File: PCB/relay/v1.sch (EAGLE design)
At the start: 7 parts, among them T1 BC817, U1 SFH615A-07, U2 ALQ105

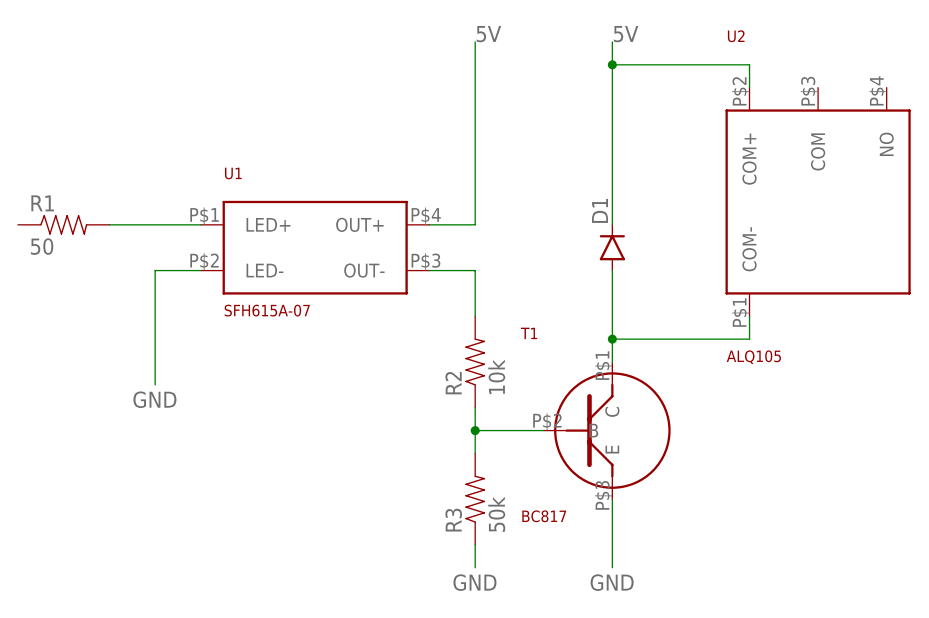
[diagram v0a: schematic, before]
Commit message: Adding files for v0.2
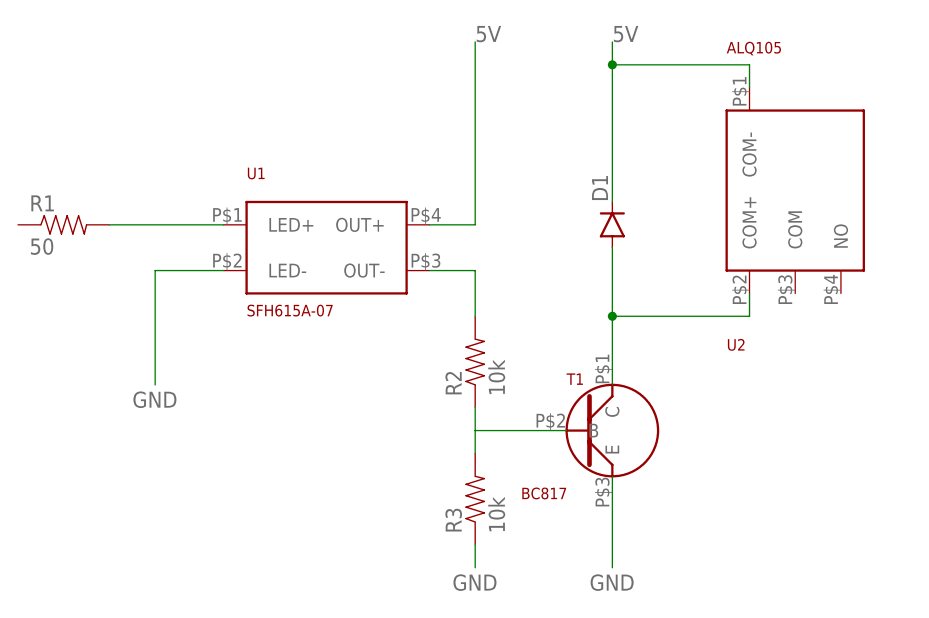
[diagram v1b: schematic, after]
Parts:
- R3: value 50k -> 10k
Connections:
- net 5V: now also U2.COM-; no longer U2.COM+
- net N$4: now also U2.COM+; no longer U2.COM-
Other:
- moved on the sheet: D1, U1, U2
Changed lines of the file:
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@@
 </classes>
 <parts>
-<part name="U1" library="lib" deviceset="SFH615A-07" device=""/>
+<part name="U1" library="lib" library_urn="urn:adsk.eagle:library:473707" deviceset="SFH615A-07" device="" package3d_urn="urn:adsk.eagle:package:473718/1"/>
 <part name="R1" library="SparkFun-Passives" deviceset="RESISTOR" device="0603-RES" value="50"/>
-<part name="T1" library="lib" deviceset="BC817" device=""/>
+<part name="T1" library="lib" library_urn="urn:adsk.eagle:library:473707" deviceset="BC817" device="" package3d_urn="urn:adsk.eagle:package:473719/1"/>
 <part name="R2" library="SparkFun-Passives" deviceset="RESISTOR" device="0603-RES" value="10k"/>
-<part name="R3" library="SparkFun-Passives" deviceset="RESISTOR" device="0603-RES" value="50k"/>
 <part name="D1" library="SparkFun-DiscreteSemi" deviceset="DIODE" device="SMA"/>
-<part name="U2" library="lib" deviceset="ALQ105" device=""/>
+<part name="U2" library="lib" library_urn="urn:adsk.eagle:library:473707" deviceset="ALQ105" device="" package3d_urn="urn:adsk.eagle:package:473720/1"/>
+<part name="R3" library="SparkFun-Passives" deviceset="RESISTOR" device="0603-RES" value="10k"/>
 </parts>
 <sheets>
@@
 <instance part="U1" gate="G$1" x="40.64" y="48.26"/>
 <instance part="R1" gate="G$1" x="12.7" y="50.8"/>
-<instance part="T1" gate="G$1" x="73.66" y="27.94"/>
+<instance part="T1" gate="G$1" x="73.66" y="27.94" smashed="yes">
+<attribute name="NAME" x="68.58" y="33.02" size="1.27" layer="94"/>
+<attribute name="VALUE" x="63.5" y="20.32" size="1.27" layer="94"/>
+</instance>
 <instance part="R2" gate="G$1" x="58.42" y="35.56" rot="R90"/>
+<instance part="D1" gate="G$1" x="73.66" y="50.8" rot="R90"/>
+<instance part="U2" gate="G$1" x="93.98" y="53.34" rot="MR180"/>
 <instance part="R3" gate="G$1" x="58.42" y="20.32" rot="R90"/>
-<instance part="D1" gate="G$1" x="73.66" y="48.26" rot="R90"/>
-<instance part="U2" gate="G$1" x="106.68" y="48.26"/>
 </instances>
 <busses>
@@
 <pinref part="R1" gate="G$1" pin="2"/>
 <pinref part="U1" gate="G$1" pin="LED+"/>
-<wire x1="17.78" y1="50.8" x2="27.94" y2="50.8" width="0.1524" layer="91"/>
+<wire x1="17.78" y1="50.8" x2="30.48" y2="50.8" width="0.1524" layer="91"/>
 </segment>
 </net>
@@
 <segment>
 <pinref part="U1" gate="G$1" pin="LED-"/>
-<wire x1="27.94" y1="45.72" x2="22.86" y2="45.72" width="0.1524" layer="91"/>
+<wire x1="30.48" y1="45.72" x2="22.86" y2="45.72" width="0.1524" layer="91"/>
 <wire x1="22.86" y1="45.72" x2="22.86" y2="33.02" width="0.1524" layer="91"/>
 <label x="20.32" y="30.48" size="1.778" layer="95"/>
+</segment>
+<segment>
+<pinref part="T1" gate="G$1" pin="E"/>
+<wire x1="73.66" y1="22.86" x2="73.66" y2="12.7" width="0.1524" layer="91"/>
+<label x="71.12" y="10.16" size="1.778" layer="95"/>
 </segment>
 <segment>
@@
 <wire x1="58.42" y1="15.24" x2="58.42" y2="12.7" width="0.1524" layer="91"/>
 <label x="55.88" y="10.16" size="1.778" layer="95"/>
-</segment>
-<segment>
-<pinref part="T1" gate="G$1" pin="E"/>
-<wire x1="73.66" y1="20.32" x2="73.66" y2="12.7" width="0.1524" layer="91"/>
-<label x="71.12" y="10.16" size="1.778" layer="95"/>
 </segment>
 </net>
@@
 <segment>
 <pinref part="R2" gate="G$1" pin="1"/>
-<pinref part="R3" gate="G$1" pin="2"/>
 <wire x1="58.42" y1="30.48" x2="58.42" y2="27.94" width="0.1524" layer="91"/>
 <pinref part="T1" gate="G$1" pin="B"/>
+<wire x1="68.58" y1="27.94" x2="58.42" y2="27.94" width="0.1524" layer="91"/>
+<pinref part="R3" gate="G$1" pin="2"/>
 <wire x1="58.42" y1="27.94" x2="58.42" y2="25.4" width="0.1524" layer="91"/>
-<wire x1="66.04" y1="27.94" x2="58.42" y2="27.94" width="0.1524" layer="91"/>
-<junction x="58.42" y="27.94"/>
 </segment>
 </net>
@@
 <segment>
 <pinref part="D1" gate="G$1" pin="C"/>
-<wire x1="73.66" y1="50.8" x2="73.66" y2="68.58" width="0.1524" layer="91"/>
+<wire x1="73.66" y1="53.34" x2="73.66" y2="68.58" width="0.1524" layer="91"/>
 <label x="73.66" y="71.12" size="1.778" layer="95"/>
-<pinref part="U2" gate="G$1" pin="COM+"/>
+<pinref part="U2" gate="G$1" pin="COM-"/>
 <wire x1="73.66" y1="68.58" x2="73.66" y2="71.12" width="0.1524" layer="91"/>
 <wire x1="88.9" y1="66.04" x2="88.9" y2="68.58" width="0.1524" layer="91"/>
@@
 <pinref part="D1" gate="G$1" pin="A"/>
 <pinref part="T1" gate="G$1" pin="C"/>
-<wire x1="73.66" y1="45.72" x2="73.66" y2="38.1" width="0.1524" layer="91"/>
-<pinref part="U2" gate="G$1" pin="COM-"/>
-<wire x1="73.66" y1="38.1" x2="73.66" y2="35.56" width="0.1524" layer="91"/>
-<wire x1="88.9" y1="40.64" x2="88.9" y2="38.1" width="0.1524" layer="91"/>
-<wire x1="88.9" y1="38.1" x2="73.66" y2="38.1" width="0.1524" layer="91"/>
-<junction x="73.66" y="38.1"/>
+<wire x1="73.66" y1="48.26" x2="73.66" y2="40.64" width="0.1524" layer="91"/>
+<pinref part="U2" gate="G$1" pin="COM+"/>
+<wire x1="73.66" y1="40.64" x2="73.66" y2="33.02" width="0.1524" layer="91"/>
+<wire x1="88.9" y1="43.18" x2="88.9" y2="40.64" width="0.1524" layer="91"/>
+<wire x1="88.9" y1="40.64" x2="73.66" y2="40.64" width="0.1524" layer="91"/>
+<junction x="73.66" y="40.64"/>
 </segment>
 </net>
@@
 </schematic>
 </drawing>
+<compatibility>
+<note version="8.2" severity="warning">
+Since Version 8.2, EAGLE supports online libraries. The ids
+of those online libraries will not be understood (or retained)
+with this version.
+</note>
+<note version="8.3" severity="warning">
+Since Version 8.3, EAGLE supports URNs for individual library
+assets (packages, symbols, and devices). The URNs of those assets
+will not be understood (or retained) with this version.
+</note>
+<note version="8.3" severity="warning">
+Since Version 8.3, EAGLE supports the association of 3D packages
+with devices in libraries, schematics, and board files. Those 3D
+packages will not be understood (or retained) with this version.
+</note>
+</compatibility>
 </eagle>
